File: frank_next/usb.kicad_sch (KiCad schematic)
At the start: 44 parts, among them J10 USB4215-03-A, J11 USB4215-03-A, J8 676430910, J9 676430910, U10 TPD4S012DRYR, U11 TPD4S012DRYR, U12 TPD4S012DRYR, U13 TPS2116DRL, U14 TS3USB221RSER, U15 AMS1117-3.3, U16 CH334F, U9 TPD4S012DRYR, Y3 12MHz

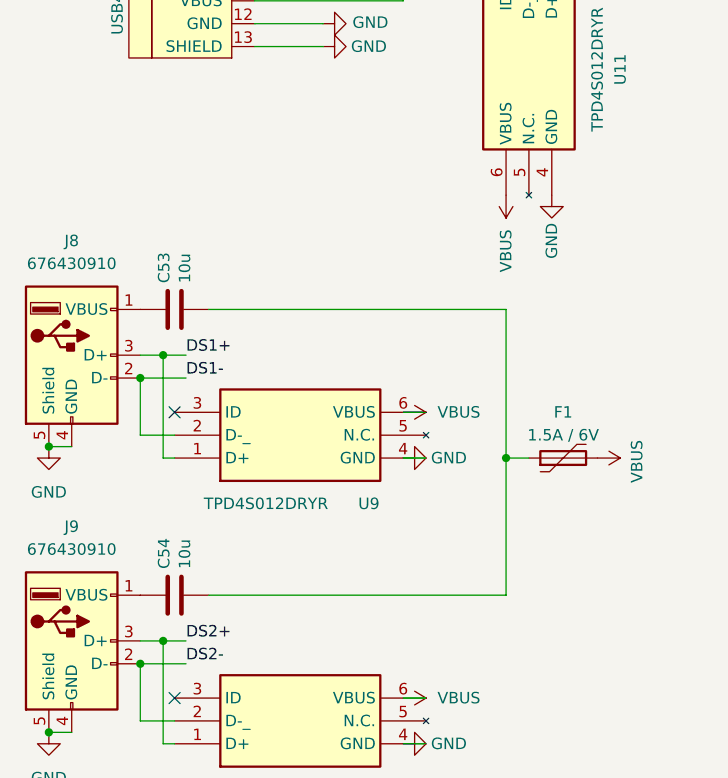
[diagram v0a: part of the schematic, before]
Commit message: Board updates
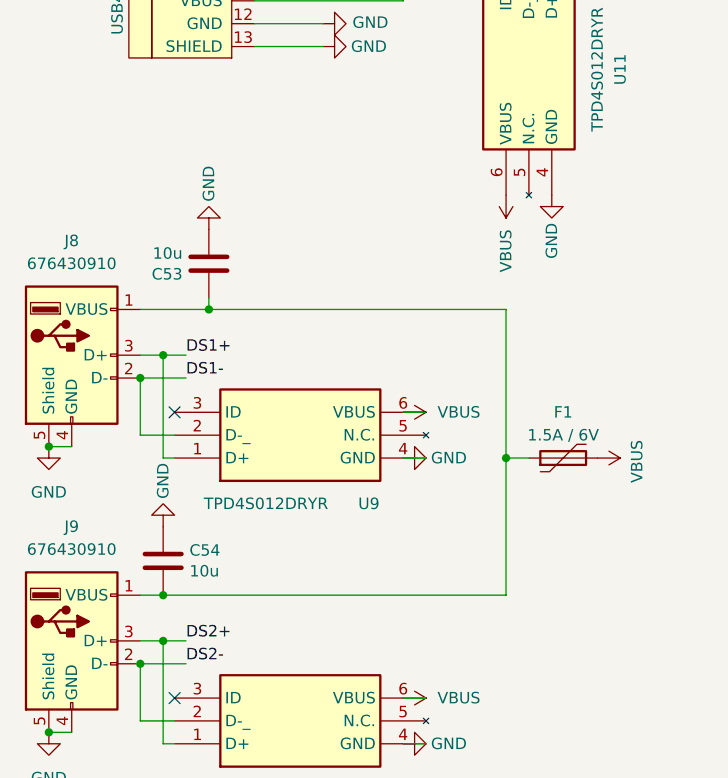
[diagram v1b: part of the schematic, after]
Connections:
- net GND: now also C53.2, C54.1
- net at C53.1, J8.1 (VBUS): now also C54.2, F1.1, J9.1 (VBUS)
